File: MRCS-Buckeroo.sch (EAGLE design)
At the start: 8 parts

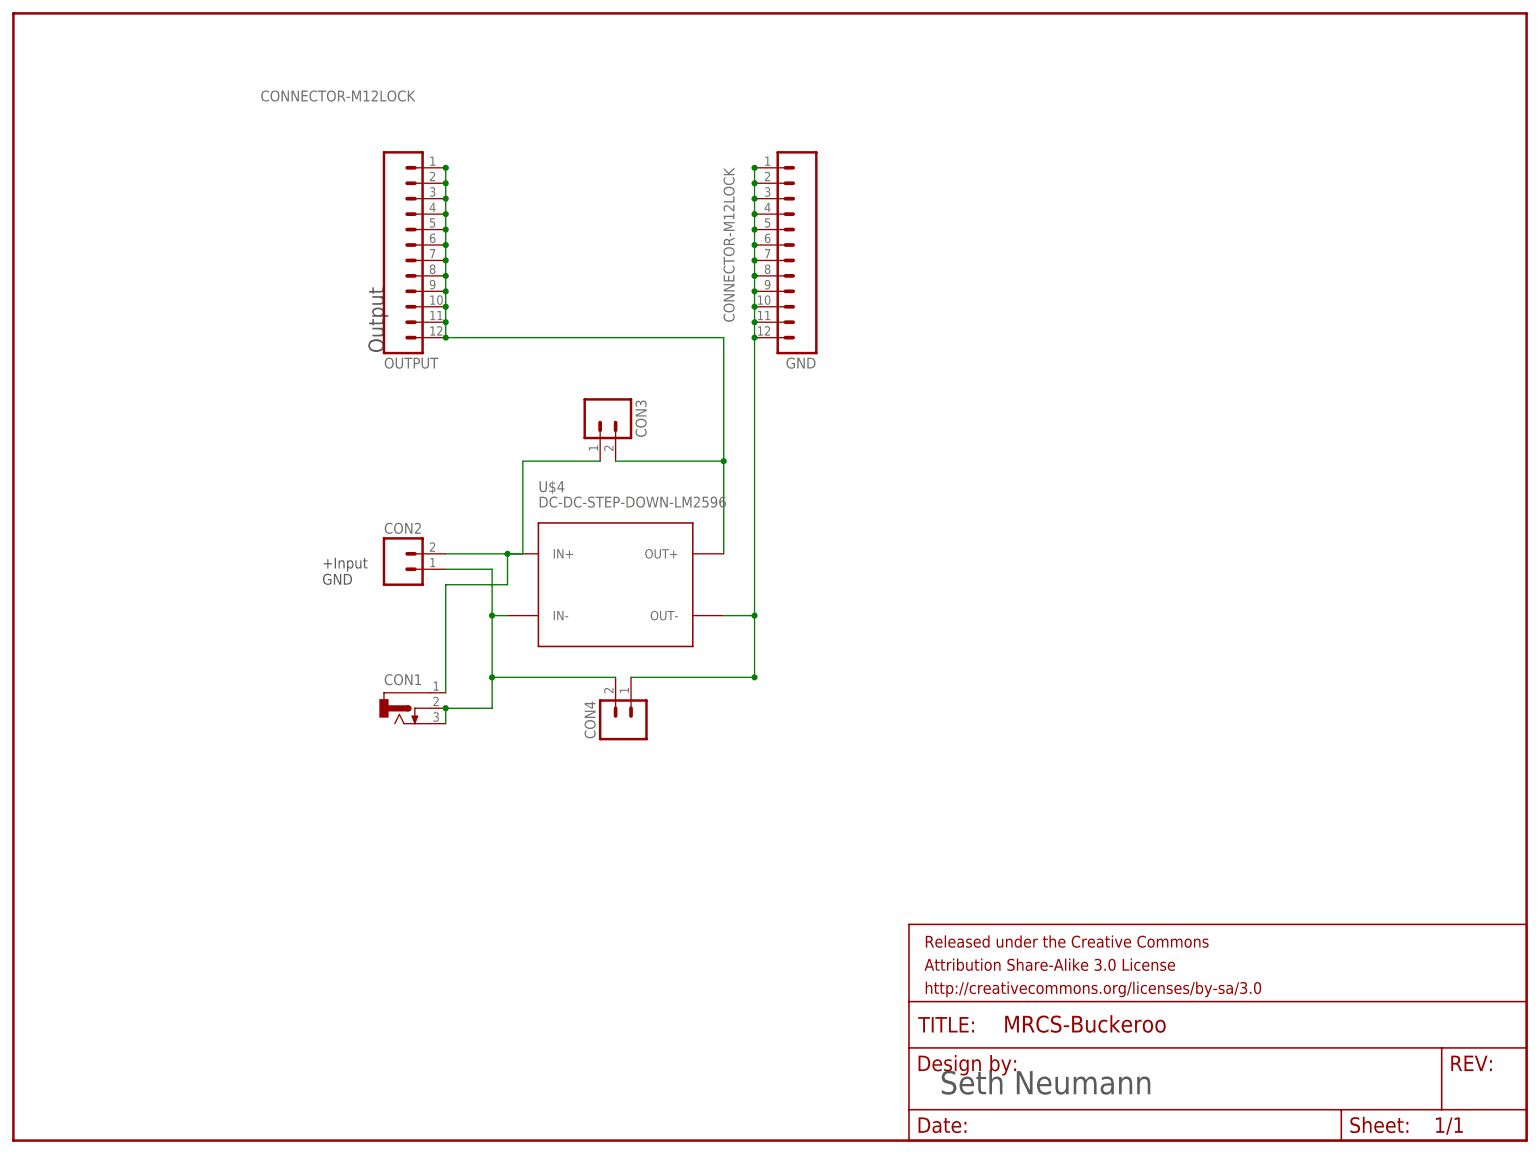
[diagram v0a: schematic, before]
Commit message: sent to fab
sent to fab
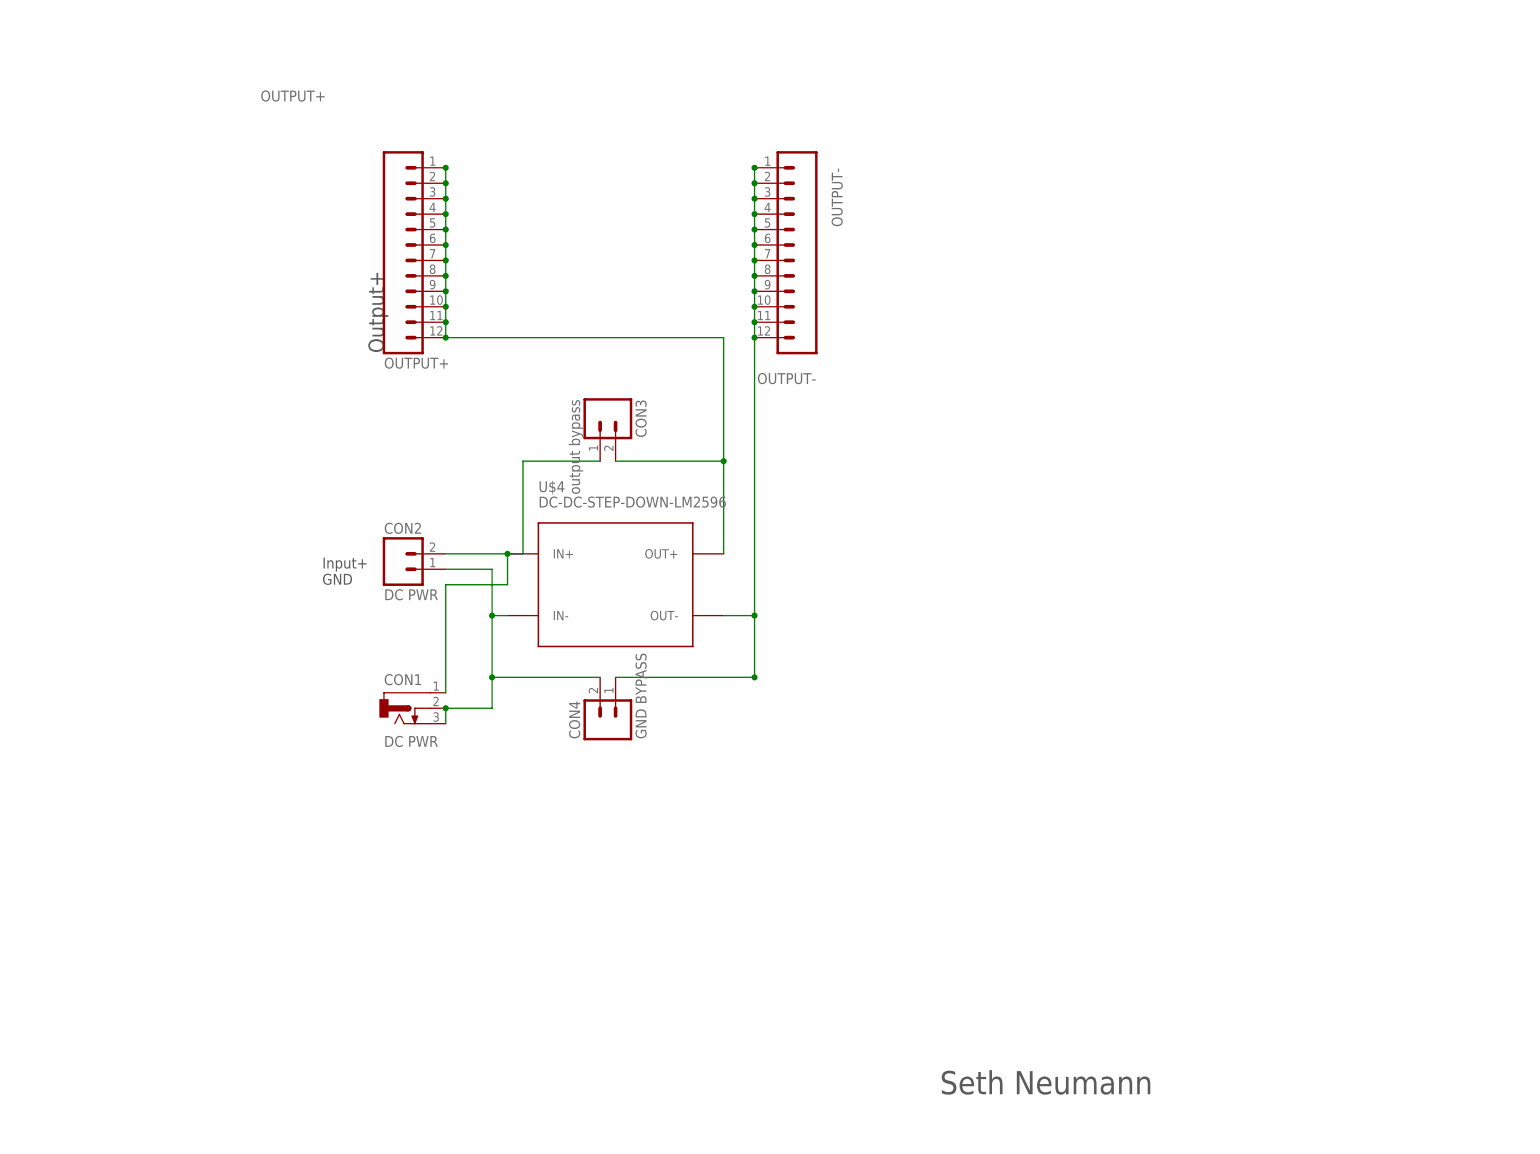
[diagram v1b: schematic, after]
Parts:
- removed FRAME1: FRAME-LETTER, SparkFun-Aesthetics:FRAME-LETTER
- CON1, CON2: value (none) -> DC PWR
- CON3: value (none) -> output bypass
- CON4: value (none) -> GND BYPASS
- OUTPUT+: value CONNECTOR-M12LOCK -> OUTPUT+
- OUTPUT-: value CONNECTOR-M12LOCK -> OUTPUT-
- renumbered GND to OUTPUT-, OUTPUT to OUTPUT+
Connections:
- net N$1 renamed INPUT+
- net N$2 renamed GND
- net N$3 renamed OUTPUT-
- net N$4 renamed OUTPUT+
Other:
- note added: "Input+ GND"
- note added: "Output+"
- note removed: "+Input GND"
- note removed: "Output"
- moved on the sheet: CON4
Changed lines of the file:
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@@
 </classes>
 <parts>
-<part name="OUTPUT" library="SPCoast" deviceset="CONNECTOR-M12" device="LOCK"/>
-<part name="GND" library="SPCoast" deviceset="CONNECTOR-M12" device="LOCK"/>
-<part name="CON1" library="SPCoast" deviceset="CONNECTOR-DC-POWER" device="-RA"/>
-<part name="CON2" library="SPCoast" deviceset="CONNECTOR-M02" device="3.5MM-LOCK"/>
+<part name="OUTPUT+" library="SPCoast" deviceset="CONNECTOR-M12" device="LOCK" value="OUTPUT+"/>
+<part name="OUTPUT-" library="SPCoast" deviceset="CONNECTOR-M12" device="LOCK" value="OUTPUT-"/>
+<part name="CON1" library="SPCoast" deviceset="CONNECTOR-DC-POWER" device="-RA" value="DC PWR"/>
+<part name="CON2" library="SPCoast" deviceset="CONNECTOR-M02" device="3.5MM-LOCK" value="DC PWR"/>
 <part name="U$4" library="diy-modules" deviceset="DC-DC-STEP-DOWN-LM2596" device=""/>
-<part name="FRAME1" library="SparkFun-Aesthetics" deviceset="FRAME-LETTER" device=""/>
-<part name="CON3" library="SPCoast" deviceset="CONNECTOR-M02" device="MOLEX-1X02-LOCK"/>
-<part name="CON4" library="SPCoast" deviceset="CONNECTOR-M02" device="MOLEX-1X02-LOCK"/>
+<part name="CON3" library="SPCoast" deviceset="CONNECTOR-M02" device="MOLEX-1X02-LOCK" value="output bypass"/>
+<part name="CON4" library="SPCoast" deviceset="CONNECTOR-M02" device="MOLEX-1X02-LOCK" value="GND BYPASS"/>
 </parts>
 <sheets>
 <sheet>
 <plain>
-<text x="119.38" y="81.28" size="2.54" layer="97" rot="R90">Output</text>
-<text x="109.22" y="43.18" size="1.778" layer="97">+Input
+<text x="119.38" y="81.28" size="2.54" layer="97" rot="R90">Output+</text>
+<text x="109.22" y="43.18" size="1.778" layer="97">Input+
 GND
 </text>
@@
 </plain>
 <instances>
-<instance part="OUTPUT" gate="G$1" x="119.38" y="96.52" smashed="yes" rot="MR180">
+<instance part="OUTPUT+" gate="G$1" x="119.38" y="96.52" smashed="yes" rot="MR180">
 <attribute name="VALUE" x="99.06" y="124.46" size="1.778" layer="96" rot="MR180"/>
 <attribute name="NAME" x="119.38" y="80.518" size="1.778" layer="95" rot="MR180"/>
 </instance>
-<instance part="GND" gate="G$1" x="190.5" y="96.52" smashed="yes" rot="R180">
-<attribute name="VALUE" x="175.26" y="111.76" size="1.778" layer="96" rot="R270"/>
-<attribute name="NAME" x="190.5" y="80.518" size="1.778" layer="95" rot="R180"/>
+<instance part="OUTPUT-" gate="G$1" x="190.5" y="96.52" smashed="yes" rot="R180">
+<attribute name="VALUE" x="193.04" y="111.76" size="1.778" layer="96" rot="R270"/>
+<attribute name="NAME" x="190.5" y="77.978" size="1.778" layer="95" rot="R180"/>
 </instance>
 <instance part="CON1" gate="J" x="121.92" y="22.86"/>
 <instance part="CON2" gate="J" x="124.46" y="45.72"/>
 <instance part="U$4" gate="G$1" x="157.48" y="43.18"/>
-<instance part="FRAME1" gate="G$1" x="58.42" y="-48.26"/>
-<instance part="FRAME1" gate="G$2" x="205.74" y="-48.26"/>
 <instance part="CON3" gate="J" x="154.94" y="68.58" rot="R270"/>
-<instance part="CON4" gate="J" x="160.02" y="22.86" rot="R90"/>
+<instance part="CON4" gate="J" x="157.48" y="22.86" rot="R90"/>
 </instances>
 <busses>
 </busses>
 <nets>
-<net name="N$3" class="1">
+<net name="OUTPUT-" class="1">
 <segment>
-<pinref part="GND" gate="G$1" pin="12"/>
+<pinref part="OUTPUT-" gate="G$1" pin="12"/>
+<wire x1="180.34" y1="27.94" x2="180.34" y2="38.1" width="0.6096" layer="91"/>
+<pinref part="OUTPUT-" gate="G$1" pin="11"/>
 <wire x1="180.34" y1="38.1" x2="180.34" y2="83.82" width="0.6096" layer="91"/>
-<pinref part="GND" gate="G$1" pin="11"/>
 <wire x1="180.34" y1="83.82" x2="180.34" y2="86.36" width="0.6096" layer="91"/>
-<pinref part="GND" gate="G$1" pin="10"/>
+<pinref part="OUTPUT-" gate="G$1" pin="10"/>
 <wire x1="180.34" y1="86.36" x2="180.34" y2="88.9" width="0.6096" layer="91"/>
-<pinref part="GND" gate="G$1" pin="9"/>
+<pinref part="OUTPUT-" gate="G$1" pin="9"/>
 <wire x1="180.34" y1="88.9" x2="180.34" y2="91.44" width="0.6096" layer="91"/>
-<pinref part="GND" gate="G$1" pin="8"/>
+<pinref part="OUTPUT-" gate="G$1" pin="8"/>
 <wire x1="180.34" y1="91.44" x2="180.34" y2="93.98" width="0.6096" layer="91"/>
-<pinref part="GND" gate="G$1" pin="7"/>
+<pinref part="OUTPUT-" gate="G$1" pin="7"/>
 <wire x1="180.34" y1="93.98" x2="180.34" y2="96.52" width="0.6096" layer="91"/>
-<pinref part="GND" gate="G$1" pin="6"/>
+<pinref part="OUTPUT-" gate="G$1" pin="6"/>
 <wire x1="180.34" y1="96.52" x2="180.34" y2="99.06" width="0.6096" layer="91"/>
-<pinref part="GND" gate="G$1" pin="5"/>
+<pinref part="OUTPUT-" gate="G$1" pin="5"/>
 <wire x1="180.34" y1="99.06" x2="180.34" y2="101.6" width="0.6096" layer="91"/>
-<pinref part="GND" gate="G$1" pin="4"/>
+<pinref part="OUTPUT-" gate="G$1" pin="4"/>
 <wire x1="180.34" y1="101.6" x2="180.34" y2="104.14" width="0.6096" layer="91"/>
-<pinref part="GND" gate="G$1" pin="3"/>
+<pinref part="OUTPUT-" gate="G$1" pin="3"/>
 <wire x1="180.34" y1="104.14" x2="180.34" y2="106.68" width="0.6096" layer="91"/>
-<pinref part="GND" gate="G$1" pin="2"/>
+<pinref part="OUTPUT-" gate="G$1" pin="2"/>
 <wire x1="180.34" y1="106.68" x2="180.34" y2="109.22" width="0.6096" layer="91"/>
-<pinref part="GND" gate="G$1" pin="1"/>
+<pinref part="OUTPUT-" gate="G$1" pin="1"/>
 <wire x1="180.34" y1="109.22" x2="180.34" y2="111.76" width="0.6096" layer="91"/>
 <junction x="180.34" y="83.82"/>
@@
 <junction x="180.34" y="111.76"/>
 <pinref part="U$4" gate="G$1" pin="OUT-"/>
-<wire x1="180.34" y1="38.1" x2="175.26" y2="38.1" width="0.6096" layer="91"/>
+<wire x1="175.26" y1="38.1" x2="180.34" y2="38.1" width="0.6096" layer="91"/>
 <pinref part="CON4" gate="J" pin="A"/>
-<wire x1="160.02" y1="27.94" x2="180.34" y2="27.94" width="0.6096" layer="91"/>
-<wire x1="180.34" y1="27.94" x2="180.34" y2="38.1" width="0.6096" layer="91"/>
+<wire x1="157.48" y1="27.94" x2="180.34" y2="27.94" width="0.6096" layer="91"/>
 <junction x="180.34" y="27.94"/>
 <junction x="180.34" y="38.1"/>
 </segment>
 </net>
-<net name="N$4" class="1">
+<net name="OUTPUT+" class="1">
 <segment>
-<pinref part="OUTPUT" gate="G$1" pin="1"/>
+<pinref part="OUTPUT+" gate="G$1" pin="1"/>
 <junction x="129.54" y="111.76"/>
-<pinref part="OUTPUT" gate="G$1" pin="2"/>
+<pinref part="OUTPUT+" gate="G$1" pin="2"/>
 <wire x1="129.54" y1="109.22" x2="129.54" y2="111.76" width="0.6096" layer="91"/>
 <junction x="129.54" y="109.22"/>
-<pinref part="OUTPUT" gate="G$1" pin="3"/>
+<pinref part="OUTPUT+" gate="G$1" pin="3"/>
 <wire x1="129.54" y1="106.68" x2="129.54" y2="109.22" width="0.6096" layer="91"/>
 <junction x="129.54" y="106.68"/>
-<pinref part="OUTPUT" gate="G$1" pin="4"/>
+<pinref part="OUTPUT+" gate="G$1" pin="4"/>
 <wire x1="129.54" y1="104.14" x2="129.54" y2="106.68" width="0.6096" layer="91"/>
-<pinref part="OUTPUT" gate="G$1" pin="5"/>
+<pinref part="OUTPUT+" gate="G$1" pin="5"/>
 <wire x1="129.54" y1="104.14" x2="129.54" y2="101.6" width="0.6096" layer="91"/>
-<pinref part="OUTPUT" gate="G$1" pin="6"/>
+<pinref part="OUTPUT+" gate="G$1" pin="6"/>
 <wire x1="129.54" y1="101.6" x2="129.54" y2="99.06" width="0.6096" layer="91"/>
-<pinref part="OUTPUT" gate="G$1" pin="7"/>
+<pinref part="OUTPUT+" gate="G$1" pin="7"/>
 <wire x1="129.54" y1="99.06" x2="129.54" y2="96.52" width="0.6096" layer="91"/>
-<pinref part="OUTPUT" gate="G$1" pin="8"/>
+<pinref part="OUTPUT+" gate="G$1" pin="8"/>
 <wire x1="129.54" y1="96.52" x2="129.54" y2="93.98" width="0.6096" layer="91"/>
-<pinref part="OUTPUT" gate="G$1" pin="12"/>
-<pinref part="OUTPUT" gate="G$1" pin="11"/>
+<pinref part="OUTPUT+" gate="G$1" pin="12"/>
+<pinref part="OUTPUT+" gate="G$1" pin="11"/>
 <wire x1="129.54" y1="83.82" x2="129.54" y2="86.36" width="0.6096" layer="91"/>
-<pinref part="OUTPUT" gate="G$1" pin="10"/>
+<pinref part="OUTPUT+" gate="G$1" pin="10"/>
 <wire x1="129.54" y1="86.36" x2="129.54" y2="88.9" width="0.6096" layer="91"/>
-<pinref part="OUTPUT" gate="G$1" pin="9"/>
+<pinref part="OUTPUT+" gate="G$1" pin="9"/>
 <wire x1="129.54" y1="88.9" x2="129.54" y2="91.44" width="0.6096" layer="91"/>
 <junction x="129.54" y="83.82"/>
@@
 </segment>
 </net>
-<net name="N$1" class="0">
+<net name="INPUT+" class="0">
 <segment>
 <pinref part="CON2" gate="J" pin="B"/>
@@
 </segment>
 </net>
-<net name="N$2" class="0">
+<net name="GND" class="0">
 <segment>
 <pinref part="CON2" gate="J" pin="A"/>
@@
 <pinref part="CON4" gate="J" pin="B"/>
 <wire x1="137.16" y1="27.94" x2="137.16" y2="38.1" width="0.6096" layer="91"/>
-<wire x1="157.48" y1="27.94" x2="137.16" y2="27.94" width="0.6096" layer="91"/>
+<wire x1="154.94" y1="27.94" x2="137.16" y2="27.94" width="0.6096" layer="91"/>
 <junction x="137.16" y="27.94"/>
 </segment>
